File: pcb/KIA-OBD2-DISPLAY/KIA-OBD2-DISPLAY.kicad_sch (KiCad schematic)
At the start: 6 parts, among them U4 CAP1188-1-CP-TR, U5 MCP2515-xSO, U6 TJA1050, U9 ESP32-C6-MINI-1/U

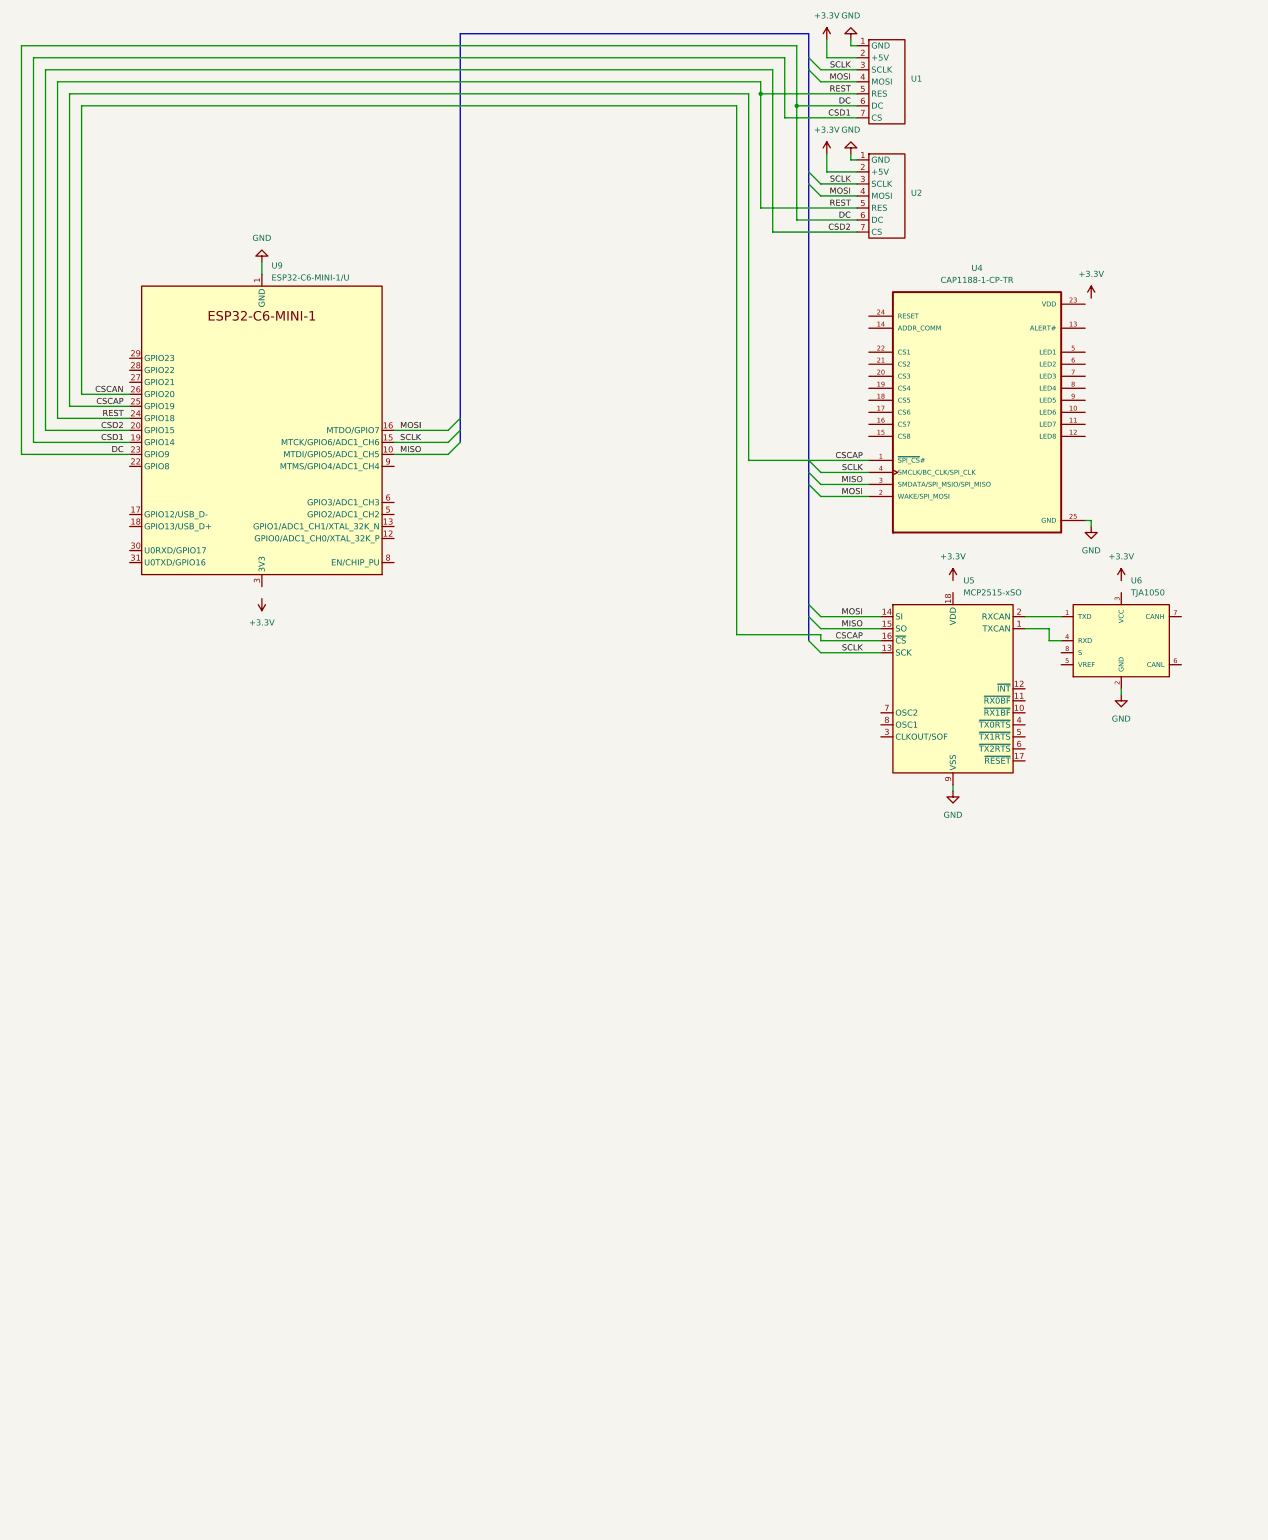
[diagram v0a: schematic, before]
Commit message: pcb 3d work
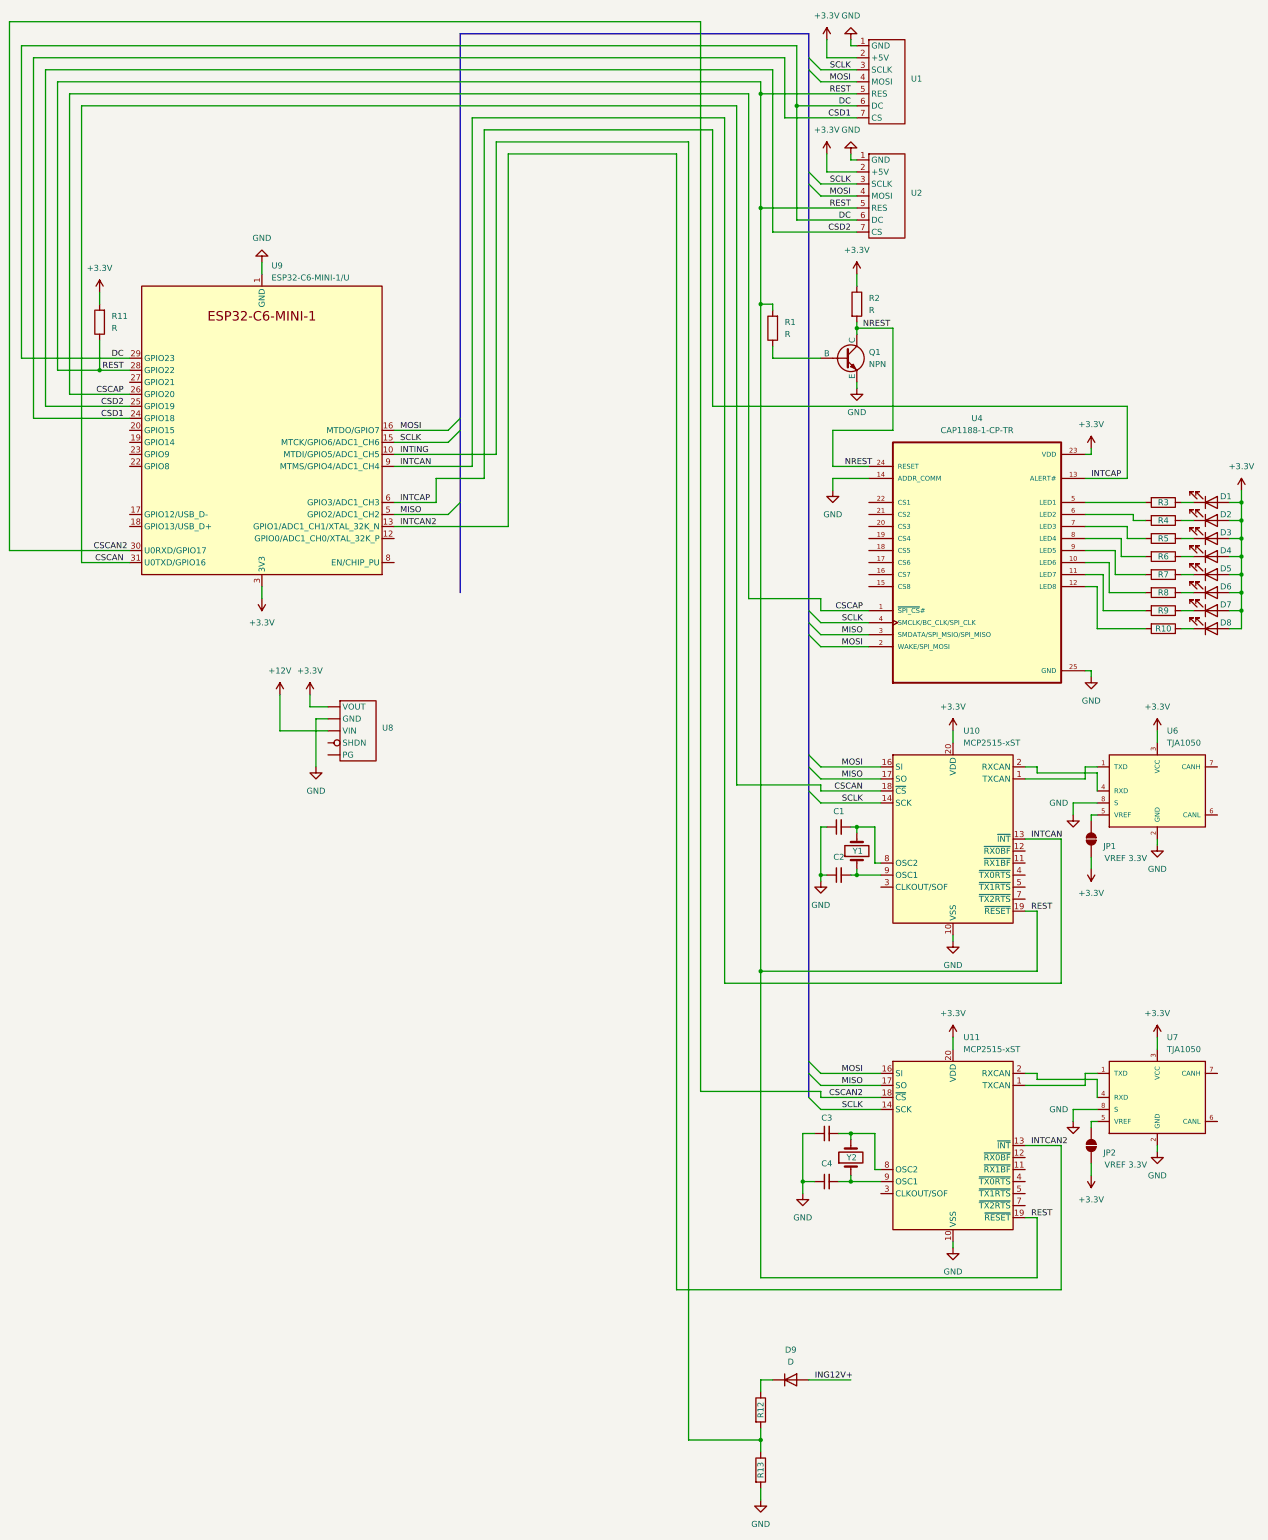
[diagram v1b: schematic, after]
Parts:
- removed U5: MCP2515-xSO, Package_SO:SOIC-18W_7.5x11.6mm_P1.27mm, symbol Interface_CAN_LIN:MCP2515-xSO
- added C1, C2, C3, C4: 22pF, symbol Device:C_Small
- added D1, D2, D3, D4, D5, D6, D7, D8: LED, symbol Device:LED
- added D9: D, symbol Device:D
- added JP1, JP2: VREF 3.3V, symbol Jumper:SolderJumper_2_Open
- added Q1: NPN, symbol Simulation_SPICE:NPN
- added R1, R10, R11, R12, R13, R2, R3, R4, R5, R6, R7, R8, R9: R, symbol Device:R
- added U10, U11: MCP2515-xST, Package_SO:TSSOP-20_4.4x6.5mm_P0.65mm, symbol Interface_CAN_LIN:MCP2515-xST
- added U7: TJA1050, TJA1050:SOT96-1, symbol TJA1050C:TJA1050
- added U8: ~, symbol D24V10F3:D24V10F3
- added Y1, Y2: Crystal, symbol Device:Crystal
- U1, U2: footprint (none) -> SH1122:SH1122
- U4: footprint CAP1188-1-CP-TR:QFN50P400X400X90-25N -> CAP1188:QFN50P400X400X90-25N
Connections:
- net +3.3V: now also U4.23 (VDD), U6.3 (VCC), U9.3 (3V3), D1.2 (A), D2.2 (A), D3.2 (A), D4.2 (A), D5.2 (A), D6.2 (A), D7.2 (A), D8.2 (A), JP1.1 (A), JP2.1 (A), R11.2, R2.1, U10.20 (VDD), U11.20 (VDD), U7.3 (VCC), U8. (VOUT)
- net CSCAN: now also U9.31 (U0TXD/GPIO16), U10.18 (~{CS}); no longer U4.1 (~{SPI_CS}#), U9.25 (GPIO19), U9.26 (GPIO20)
- net CSD1: now also U9.24 (GPIO18); no longer U9.19 (GPIO14)
- net CSD2: now also U9.25 (GPIO19); no longer U9.20 (GPIO15)
- net DC: now also U9.29 (GPIO23); no longer U9.23 (GPIO9)
- net GND: now also U4.14 (ADDR_COMM), U6.8 (S), C1.1, C2.1, C3.1, C4.1, Q1.3 (E), R13.2, U10.10 (VSS), U11.10 (VSS), U7.2 (GND), U7.8 (S), U8. (VOUT)
- net MISO: now also U9.5 (GPIO2/ADC1_CH2), U10.17 (SO), U11.17 (SO); no longer U9.10 (MTDI/GPIO5/ADC1_CH5)
- net MOSI: now also U10.16 (SI), U11.16 (SI)
- net REST: now also U9.28 (GPIO22), R1.2, R11.1, U10.19 (~{RESET}), U11.19 (~{RESET}); no longer U9.24 (GPIO18)
- net SCLK: now also U10.14 (SCK), U11.14 (SCK)
- net at U4.10 (LED6): now also R8.2
- net at U4.11 (LED7): now also R9.2
- net at U4.12 (LED8): now also R10.2
- net INTCAP: now reaches U4.13 (ALERT#)
- net INTCAP: now also U9.6 (GPIO3/ADC1_CH3)
- net NREST: now reaches U4.24 (RESET)
- net NREST: now also Q1.1 (C), R2.2
- net at U4.5 (LED1): now also R3.2
- net at U4.6 (LED2): now also R4.2
- net at U4.7 (LED3): now also R5.2
- net at U4.8 (LED4): now also R6.2
- net at U4.9 (LED5): now also R7.2
- net INTCAN2: now reaches U9.13 (GPIO1/ADC1_CH1/XTAL_32K_N)
- net INTCAN2: now also U11.13 (~{INT})
- net CSCAN2: now reaches U9.30 (U0RXD/GPIO17)
- net CSCAN2: now also U11.18 (~{CS})
- net INTCAN: now reaches U9.9 (MTMS/GPIO4/ADC1_CH4)
- net INTCAN: now also U10.13 (~{INT})
- net at U6.1 (TXD): now also U10.1 (TXCAN)
- net at U6.4 (RXD): now also U10.2 (RXCAN)
- net at U6.5 (VREF): now also JP1.2 (B)
- new net: C2.2, U10.9 (OSC1), Y1.1
- new net: D8.1 (K), R10.1
- new net: U11.1 (TXCAN), U7.1 (TXD)
- new net: U11.2 (RXCAN), U7.4 (RXD)
- new net: C3.2, U11.8 (OSC2), Y2.2
- new net: C4.2, U11.9 (OSC1), Y2.1
- new net: D5.1 (K), R7.1
- new net: JP2.2 (B), U7.5 (VREF)
- new net: D9.1 (K), R12.1
- new net: D2.1 (K), R4.1
- new net: D4.1 (K), R6.1
- new net: D7.1 (K), R9.1
- new net: Q1.2 (B), R1.1
- new net: D6.1 (K), R8.1
- new net: D1.1 (K), R3.1
- new net: D3.1 (K), R5.1
- new net: C1.2, U10.8 (OSC2), Y1.2
- new net +12V: U8. (VOUT)
- new net CSCAP: U4.1 (~{SPI_CS}#), U9.26 (GPIO20)
- new net ING12V+: D9.2 (A)
- new net INTING: R12.2, R13.1, U9.10 (MTDI/GPIO5/ADC1_CH5)
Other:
- moved on the sheet: U4, U6
